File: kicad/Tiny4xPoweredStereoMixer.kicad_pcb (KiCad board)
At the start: 4 copper layers, 99.1 x 56.5 mm, 58 parts, among them J1 AudioJack3_SwitchTR, J2 AudioJack3_SwitchTR, J3 AudioJack3_SwitchTR, J4 AudioJack3_SwitchTR, J6 PowerConnector, J7 PowerConnector, J8 PowerConnector, J9 AudioJack3_SwitchTR, U1 TL072, U2 TL072, U6 LM2611AMF/NOPB

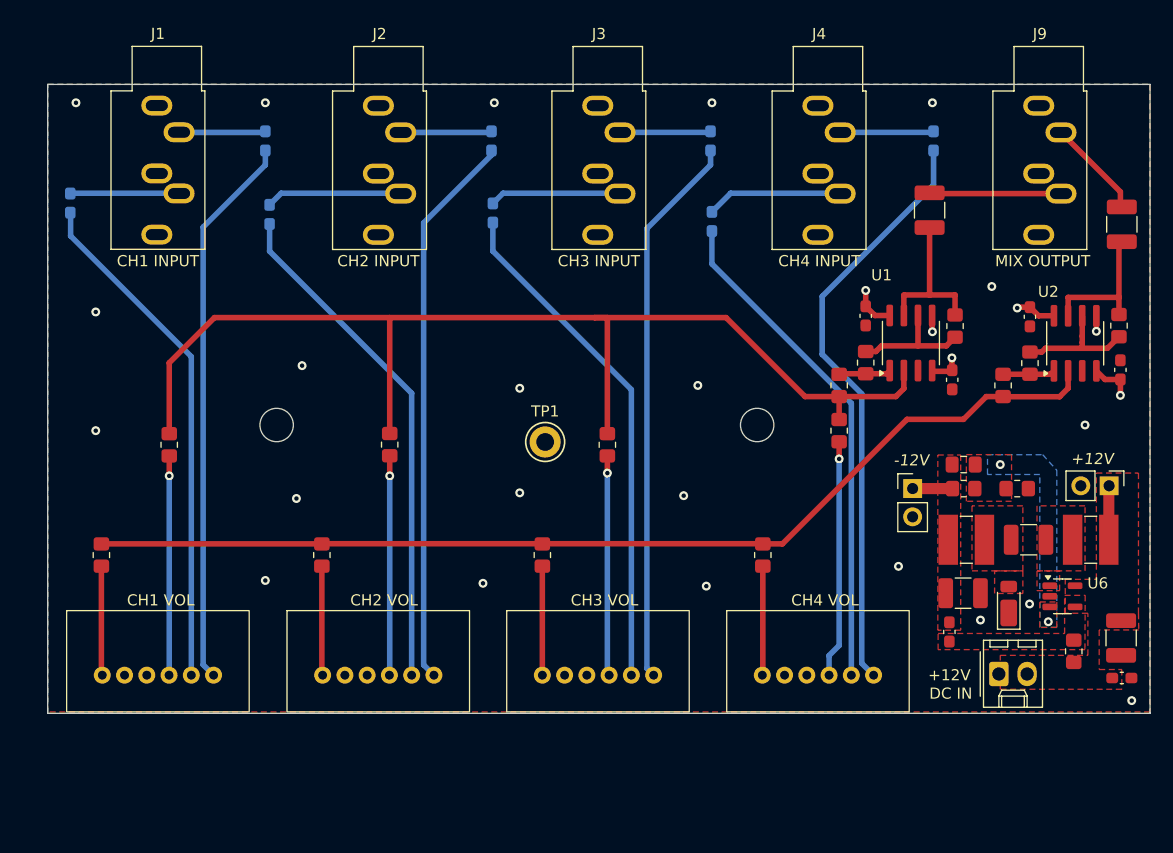
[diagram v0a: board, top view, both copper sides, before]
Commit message: updated main
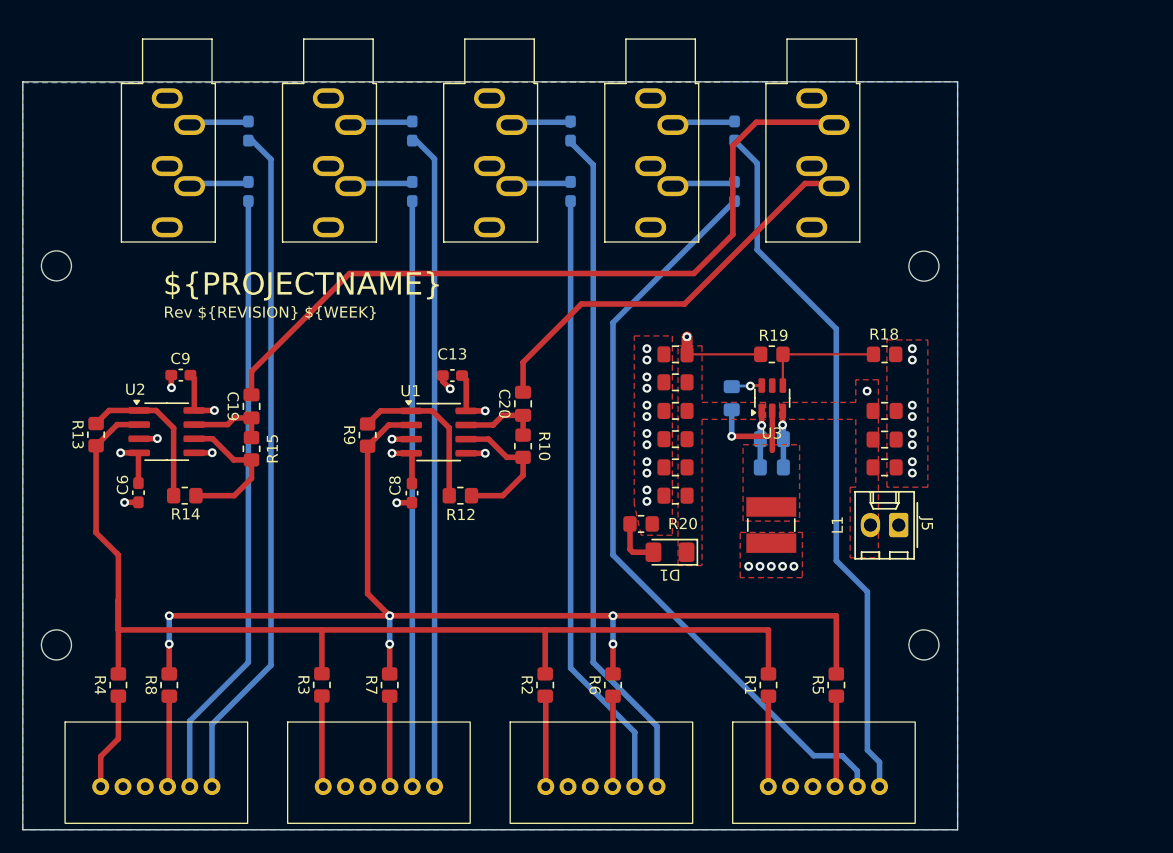
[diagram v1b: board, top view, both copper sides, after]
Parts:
- removed J6: PowerConnector, Connector_Molex:Molex_KK-254_AE-6410-02A_1x02_P2.54mm_Vertical
- removed J7, J8: PowerConnector, Connector_PinHeader_2.54mm:PinHeader_1x02_P2.54mm_Vertical
- removed L2: 22u, Inductor_SMD:L_Ferrocore_DLG-0403
- removed R11: 100k, Resistor_SMD:R_0805_2012Metric_Pad1.20x1.40mm_HandSolder
- removed RFB1: 22k, Resistor_SMD:R_0805_2012Metric_Pad1.20x1.40mm_HandSolder
- removed RFB2: 2k2, Resistor_SMD:R_0805_2012Metric_Pad1.20x1.40mm_HandSolder
- removed TP1: TestPoint, TestPoint:TestPoint_Keystone_5005-5009_Compact
- removed U6: LM2611AMF/NOPB, Package_TO_SOT_SMD:SOT-23-5
- added C21: 100nF, Capacitor_SMD:C_0805_2012Metric_Pad1.18x1.45mm_HandSolder, F.Cu at (160.3, 85.1)
- added C22: 22uF, Capacitor_SMD:C_0805_2012Metric_Pad1.18x1.45mm_HandSolder, F.Cu at (160.3, 87.6)
- added C23: 22uF, Capacitor_SMD:C_0805_2012Metric_Pad1.18x1.45mm_HandSolder, F.Cu at (160.3, 74.9)
- added C24: 22uF, Capacitor_SMD:C_0805_2012Metric_Pad1.18x1.45mm_HandSolder, F.Cu at (160.3, 77.4)
- added C25: 22uF, Capacitor_SMD:C_0805_2012Metric_Pad1.18x1.45mm_HandSolder, F.Cu at (160.3, 80.0)
- added C26: 22uF, Capacitor_SMD:C_0805_2012Metric_Pad1.18x1.45mm_HandSolder, F.Cu at (160.3, 82.5)
- added H3: MountingHole, MountingHole:MountingHole_2.7mm_M2.5, F.Cu at (104.7, 101.0)
- added H4: MountingHole, MountingHole:MountingHole_2.7mm_M2.5, F.Cu at (182.6, 101.0)
- added J5: PowerConnector, Connector_Molex:Molex_KK-254_AE-6410-02A_1x02_P2.54mm_Vertical, F.Cu at (180.4, 90.3)
- added R18: 50K, Resistor_SMD:R_0805_2012Metric_Pad1.20x1.40mm_HandSolder, F.Cu at (179.1, 74.9)
- added R19: 2K4, Resistor_SMD:R_0805_2012Metric_Pad1.20x1.40mm_HandSolder, F.Cu at (169.0, 74.9)
- added R20: 2K2, Resistor_SMD:R_0805_2012Metric_Pad1.20x1.40mm_HandSolder, F.Cu at (157.2, 90.2)
- added U3: TPS54202DDC, Package_TO_SOT_SMD:SOT-23-6, F.Cu at (169.0, 78.9)
- C1: value 22u -> 10uF; footprint Capacitor_SMD:C_1210_3225Metric_Pad1.33x2.70mm_HandSolder -> Capacitor_SMD:C_0805_2012Metric_Pad1.18x1.45mm_HandSolder
- C15: value 100nF -> 10uF; footprint Capacitor_SMD:C_0603_1608Metric_Pad1.08x0.95mm_HandSolder -> Capacitor_SMD:C_0805_2012Metric_Pad1.18x1.45mm_HandSolder; moved to B.Cu
- C16: footprint Capacitor_SMD:C_0603_1608Metric_Pad1.08x0.95mm_HandSolder -> Capacitor_SMD:C_0805_2012Metric_Pad1.18x1.45mm_HandSolder; moved to B.Cu
- C19, C20: footprint Capacitor_SMD:C_1210_3225Metric_Pad1.33x2.70mm_HandSolder -> Capacitor_SMD:C_0805_2012Metric_Pad1.18x1.45mm_HandSolder
- C2: value 2.2u -> 10uF; footprint Capacitor_SMD:C_1210_3225Metric_Pad1.33x2.70mm_HandSolder -> Capacitor_SMD:C_0805_2012Metric_Pad1.18x1.45mm_HandSolder
- C3: value 1n -> 100nF
- C4: value 22u -> 100nF; footprint Capacitor_SMD:C_1210_3225Metric_Pad1.33x2.70mm_HandSolder -> Capacitor_SMD:C_0805_2012Metric_Pad1.18x1.45mm_HandSolder; moved to B.Cu
- D1: value D_Schottky -> LED; footprint Diode_SMD:D_PowerDI-123 -> LED_SMD:LED_1206_3216Metric_Pad1.42x1.75mm_HandSolder
- H1, H2: footprint MountingHole:MountingHole_3mm -> MountingHole:MountingHole_2.7mm_M2.5
- L1: value 22u -> 22uH
- moved U2 82.0 mm to (114.6, 81.9), turned to 0 degrees
- moved R13 81.6 mm to (108.2, 82.1)
- moved C19 79.9 mm to (122.2, 79.6)
- moved R15 78.7 mm to (122.2, 83.4)
- moved R14 76.9 mm to (116.2, 87.6), turned to 0 degrees
- moved C6 73.8 mm to (112.0, 87.4)
- moved C8 64.6 mm to (136.6, 87.4), turned to -90 degrees
- moved C9 61.8 mm to (115.9, 76.8), turned to 180 degrees
- moved C13 52.2 mm to (140.3, 76.8), turned to 180 degrees
- moved U1 43.2 mm to (139.0, 81.9), turned to 0 degrees
- moved R9 42.6 mm to (132.6, 82.2)
- moved C20 40.5 mm to (146.6, 79.4)
- moved R10 40.3 mm to (146.6, 83.2)
- moved R12 38.3 mm to (141.0, 87.6), turned to 0 degrees
- moved C15 38.1 mm to (169.0, 82.5), turned to 180 degrees
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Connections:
- C1 pad 1: GND -> +12V
- C1 pad 2: Net-(J6-Pin_2) -> GND
- C15 pad 1: Net-(J6-Pin_2) -> +12V
- C15 pad 2: GND -> -12V
- C16 pad 1: Net-(J8-Pin_1) -> Net-(U3-BOOT)
- C16 pad 2: Net-(U6-~{SHDN}) -> Net-(U3-SW)
- C2 pad 1: Net-(U6-SW) -> +12V
- C2 pad 2: Net-(D1-A) -> GND
- C3 pad 1: Net-(U6-NFB) -> +12V
- C3 pad 2: Net-(J8-Pin_1) -> GND
- C4 pad 1: GND -> +12V
- C4 pad 2: Net-(J8-Pin_1) -> -12V
- D1 pad 1: GND -> -12V
- L1 pad 1: Net-(J6-Pin_2) -> Net-(U3-SW)
- L1 pad 2: Net-(U6-SW) -> GND
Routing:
- net Net-(C19-Pad2): track 8.96 -> 68.4 mm
- net Net-(C20-Pad2): track 11.7 -> 37.3 mm
- net Net-(C18-Pad2): track 45.1 -> 68.1 mm
- net -12V: track 6.95 -> 22.2 mm, vias 2 -> 4
- net /ch4_right_mix_in: track 21.3 -> 8.52 mm, vias 1 -> 0
- net Net-(C12-Pad2): track 49.8 -> 61.6 mm
- net Net-(C5-Pad2): track 49.8 -> 61.6 mm
- net /ch3_right_mix_in: track 19.8 -> 8.49 mm, vias 1 -> 0
- net /ch2_right_mix_in: track 19.7 -> 8.49 mm, vias 1 -> 0
- net /ch1_right_mix_in: track 19.7 -> 8.54 mm, vias 1 -> 0
- net /TPS54202 Inverting PSU/VSENSE: track 0.00 -> 10.9 mm
- net Net-(C17-Pad2): track 53.2 -> 63.8 mm
- net Net-(R12-Pad1): track 4.68 -> 14.5 mm
- net Net-(U3-SW): track 0.00 -> 9.59 mm, vias 0 -> 1
- net Net-(C14-Pad2): track 45.8 -> 55.4 mm
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- added copper zone on F.Cu, net +12V
- added copper zone on F.Cu, net -12V
- added copper zone on F.Cu, net Net-(U3-SW)
- removed copper zone on F.Cu, net Net-(D1-A)
- removed copper zone on F.Cu, net Net-(J6-Pin_2)
- removed copper zone on F.Cu, net Net-(J8-Pin_1)
- removed copper zone on B.Cu, net Net-(U6-NFB)
- removed copper zone on F.Cu, net Net-(U6-NFB)
- removed copper zone on F.Cu, net Net-(U6-SW)
- removed copper zone on F.Cu, net Net-(U6-~{SHDN})
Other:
- board size 99.1 x 56.5 mm -> 84 x 67.2 mm
- board text added: "${PROJECTNAME}"
- board text added: "Enclosure: https://www.hammfg.com/files/parts/pdf/RM2005S.pdf"
- board text added: "Rev ${REVISION} ${WEEK}"
- board text removed: "Tiny 4-Channel Active Stereo Mixer Rev${REVISION} ${ISSUE_DATE}"

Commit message: changed voltage rails to +/-5V; changed PSU feedback resistor to provide -5V
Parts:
- R19: value 2K4 -> 6K8
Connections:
- net +12V renamed +5V
- net -12V renamed -5V
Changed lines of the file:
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@@
 	(property "WEEK" "43/24")
 	(net 0 "")
-	(net 1 "+12V")
+	(net 1 "+5V")
 	(net 2 "GND")
-	(net 3 "-12V")
+	(net 3 "-5V")
 	(net 4 "Net-(C5-Pad2)")
 	(net 5 "Net-(C5-Pad1)")
@@
 			(layers "F.Cu" "F.Paste" "F.Mask")
 			(roundrect_rratio 0.25)
-			(net 3 "-12V")
+			(net 3 "-5V")
 			(pinfunction "V-")
 			(pintype "power_in")
@@
 			(layers "F.Cu" "F.Paste" "F.Mask")
 			(roundrect_rratio 0.25)
-			(net 1 "+12V")
+			(net 1 "+5V")
 			(pinfunction "V+")
 			(pintype "power_in")
@@
 			(layers "F.Cu" "F.Paste" "F.Mask")
 			(roundrect_rratio 0.212766)
-			(net 1 "+12V")
+			(net 1 "+5V")
 			(pintype "passive")
 		)
@@
 			(layers "F.Cu" "F.Paste" "F.Mask")
 			(roundrect_rratio 0.25)
-			(net 1 "+12V")
+			(net 1 "+5V")
 			(pintype "passive")
 		)
@@
 			(layers "F.Cu" "F.Paste" "F.Mask")
 			(roundrect_rratio 0.25)
-			(net 1 "+12V")
+			(net 1 "+5V")
 			(pintype "passive")
 		)
@@
 			(layers "F.Cu" "F.Paste" "F.Mask")
 			(roundrect_rratio 0.212766)
-			(net 3 "-12V")
+			(net 3 "-5V")
 			(pintype "passive")
 		)
@@
 			(layers "F.Cu" "F.Paste" "F.Mask")
 			(roundrect_rratio 0.212766)
-			(net 3 "-12V")
+			(net 3 "-5V")
 			(pintype "passive")
 		)
@@
 			(layers "F.Cu" "F.Paste" "F.Mask")
 			(roundrect_rratio 0.25)
-			(net 3 "-12V")
+			(net 3 "-5V")
 			(pinfunction "GND")
 			(pintype "power_in")
@@
 			(layers "F.Cu" "F.Paste" "F.Mask")
 			(roundrect_rratio 0.25)
-			(net 1 "+12V")
+			(net 1 "+5V")
 			(pinfunction "VIN")
 			(pintype "power_in")
@@
 			(layers "F.Cu" "F.Paste" "F.Mask")
 			(roundrect_rratio 0.25)
-			(net 3 "-12V")
+			(net 3 "-5V")
 			(pintype "passive")
 		)
@@
 			)
 		)
-		(property "Value" "2K4"
+		(property "Value" "6K8"
 			(at 0 1.65 0)
 			(layer "F.Fab")
@@
 			(layers "F.Cu" "F.Paste" "F.Mask")
 			(roundrect_rratio 0.208333)
-			(net 3 "-12V")
+			(net 3 "-5V")
 			(pintype "passive")
 		)
@@
 			(layers "F.Cu" "F.Paste" "F.Mask")
 			(roundrect_rratio 0.212766)
-			(net 3 "-12V")
+			(net 3 "-5V")
 			(pintype "passive")
 		)
@@
 			(layers "F.Cu" "F.Paste" "F.Mask")
 			(roundrect_rratio 0.212766)
-			(net 1 "+12V")
+			(net 1 "+5V")
 			(pintype "passive")
 		)
@@
 			(layers "F.Cu" "F.Paste" "F.Mask")
 			(roundrect_rratio 0.212766)
-			(net 3 "-12V")
+			(net 3 "-5V")
 			(pintype "passive")
 		)
@@
 			(layers "F.Cu" "F.Paste" "F.Mask")
 			(roundrect_rratio 0.212766)
-			(net 3 "-12V")
+			(net 3 "-5V")
 			(pintype "passive")
 		)
@@
 			(layers "*.Cu" "*.Mask")
 			(remove_unused_layers no)
-			(net 1 "+12V")
+			(net 1 "+5V")
 			(pinfunction "Pin_2")
 			(pintype "passive")
@@
 			)
 		)
-		(property "Mouser" "688-RK12L1210C1K "
+		(property "Mouser" "688-RK12L12A0C0R "
 			(at 0 0 0)
 			(unlocked yes)
@@
 			(layers "F.Cu" "F.Paste" "F.Mask")
 			(roundrect_rratio 0.212766)
-			(net 1 "+12V")
+			(net 1 "+5V")
 			(pintype "passive")
 		)
@@
 			(layers "F.Cu" "F.Paste" "F.Mask")
 			(roundrect_rratio 0.25)
-			(net 3 "-12V")
+			(net 3 "-5V")
 			(pintype "passive")
 		)
@@
 			(layers "F.Cu" "F.Paste" "F.Mask")
 			(roundrect_rratio 0.175439)
-			(net 3 "-12V")
+			(net 3 "-5V")
 			(pinfunction "K")
 			(pintype "passive")
@@
 			)
 		)
-		(property "Mouser" "688-RK12L1210C1K "
+		(property "Mouser" "688-RK12L12A0C0R "
 			(at 0 0 0)
 			(unlocked yes)
@@
 			(layers "F.Cu" "F.Paste" "F.Mask")
 			(roundrect_rratio 0.25)
-			(net 3 "-12V")
+			(net 3 "-5V")
 			(pinfunction "V-")
 			(pintype "power_in")
@@
 			(layers "F.Cu" "F.Paste" "F.Mask")
 			(roundrect_rratio 0.25)
-			(net 1 "+12V")
+			(net 1 "+5V")
 			(pinfunction "V+")
 			(pintype "power_in")
@@
 			)
 		)
-		(property "Mouser" "688-RK12L1210C1K "
+		(property "Mouser" "688-RK12L12A0C0R "
 			(at 0 0 0)
 			(unlocked yes)
@@
 			(layers "F.Cu" "F.Paste" "F.Mask")
 			(roundrect_rratio 0.212766)
-			(net 3 "-12V")
+			(net 3 "-5V")
 			(pintype "passive")
 		)
@@
 			)
 		)
-		(property "Mouser" "688-RK12L1210C1K "
+		(property "Mouser" "688-RK12L12A0C0R "
 			(at 0 0 0)
 			(unlocked yes)
@@
 			(layers "B.Cu" "B.Paste" "B.Mask")
 			(roundrect_rratio 0.212766)
-			(net 1 "+12V")
+			(net 1 "+5V")
 			(pintype "passive")
 		)
@@
 			(layers "B.Cu" "B.Paste" "B.Mask")
 			(roundrect_rratio 0.212766)
-			(net 3 "-12V")
+			(net 3 "-5V")
 			(pintype "passive")
 		)
@@
 			(layers "B.Cu" "B.Paste" "B.Mask")
 			(roundrect_rratio 0.212766)
-			(net 1 "+12V")
+			(net 1 "+5V")
 			(pintype "passive")
 		)
@@
 			(layers "B.Cu" "B.Paste" "B.Mask")
 			(roundrect_rratio 0.212766)
-			(net 3 "-12V")
+			(net 3 "-5V")
 			(pintype "passive")
 		)
@@
 	(zone
 		(net 3)
-		(net_name "-12V")
+		(net_name "-5V")
 		(layer "F.Cu")
 		(hatch edge 0.5)
@@
 	(zone
 		(net 1)
-		(net_name "+12V")
+		(net_name "+5V")
 		(layer "F.Cu")
 		(hatch edge 0.5)
@@
 	(zone
 		(net 1)
-		(net_name "+12V")
+		(net_name "+5V")
 		(layer "In1.Cu")
 		(hatch edge 0.5)
@@
 	(zone
 		(net 3)
-		(net_name "-12V")
+		(net_name "-5V")
 		(layer "In2.Cu")
 		(hatch edge 0.5)

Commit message: Revert "changed voltage rails to +/-5V; changed PSU feedback resistor to provide -5V"
This reverts commit 87719da26a309bbde2d2f76146bcb1e510287c62.
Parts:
- R19: value 6K8 -> 2K4
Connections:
- net +5V renamed +12V
- net -5V renamed -12V
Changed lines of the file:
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@@
 	(property "WEEK" "43/24")
 	(net 0 "")
-	(net 1 "+5V")
+	(net 1 "+12V")
 	(net 2 "GND")
-	(net 3 "-5V")
+	(net 3 "-12V")
 	(net 4 "Net-(C5-Pad2)")
 	(net 5 "Net-(C5-Pad1)")
@@
 			(layers "F.Cu" "F.Paste" "F.Mask")
 			(roundrect_rratio 0.25)
-			(net 3 "-5V")
+			(net 3 "-12V")
 			(pinfunction "V-")
 			(pintype "power_in")
@@
 			(layers "F.Cu" "F.Paste" "F.Mask")
 			(roundrect_rratio 0.25)
-			(net 1 "+5V")
+			(net 1 "+12V")
 			(pinfunction "V+")
 			(pintype "power_in")
@@
 			(layers "F.Cu" "F.Paste" "F.Mask")
 			(roundrect_rratio 0.212766)
-			(net 1 "+5V")
+			(net 1 "+12V")
 			(pintype "passive")
 		)
@@
 			(layers "F.Cu" "F.Paste" "F.Mask")
 			(roundrect_rratio 0.25)
-			(net 1 "+5V")
+			(net 1 "+12V")
 			(pintype "passive")
 		)
@@
 			(layers "F.Cu" "F.Paste" "F.Mask")
 			(roundrect_rratio 0.25)
-			(net 1 "+5V")
+			(net 1 "+12V")
 			(pintype "passive")
 		)
@@
 			(layers "F.Cu" "F.Paste" "F.Mask")
 			(roundrect_rratio 0.212766)
-			(net 3 "-5V")
+			(net 3 "-12V")
 			(pintype "passive")
 		)
@@
 			(layers "F.Cu" "F.Paste" "F.Mask")
 			(roundrect_rratio 0.212766)
-			(net 3 "-5V")
+			(net 3 "-12V")
 			(pintype "passive")
 		)
@@
 			(layers "F.Cu" "F.Paste" "F.Mask")
 			(roundrect_rratio 0.25)
-			(net 3 "-5V")
+			(net 3 "-12V")
 			(pinfunction "GND")
 			(pintype "power_in")
@@
 			(layers "F.Cu" "F.Paste" "F.Mask")
 			(roundrect_rratio 0.25)
-			(net 1 "+5V")
+			(net 1 "+12V")
 			(pinfunction "VIN")
 			(pintype "power_in")
@@
 			(layers "F.Cu" "F.Paste" "F.Mask")
 			(roundrect_rratio 0.25)
-			(net 3 "-5V")
+			(net 3 "-12V")
 			(pintype "passive")
 		)
@@
 			)
 		)
-		(property "Value" "6K8"
+		(property "Value" "2K4"
 			(at 0 1.65 0)
 			(layer "F.Fab")
@@
 			(layers "F.Cu" "F.Paste" "F.Mask")
 			(roundrect_rratio 0.208333)
-			(net 3 "-5V")
+			(net 3 "-12V")
 			(pintype "passive")
 		)
@@
 			(layers "F.Cu" "F.Paste" "F.Mask")
 			(roundrect_rratio 0.212766)
-			(net 3 "-5V")
+			(net 3 "-12V")
 			(pintype "passive")
 		)
@@
 			(layers "F.Cu" "F.Paste" "F.Mask")
 			(roundrect_rratio 0.212766)
-			(net 1 "+5V")
+			(net 1 "+12V")
 			(pintype "passive")
 		)
@@
 			(layers "F.Cu" "F.Paste" "F.Mask")
 			(roundrect_rratio 0.212766)
-			(net 3 "-5V")
+			(net 3 "-12V")
 			(pintype "passive")
 		)
@@
 			(layers "F.Cu" "F.Paste" "F.Mask")
 			(roundrect_rratio 0.212766)
-			(net 3 "-5V")
+			(net 3 "-12V")
 			(pintype "passive")
 		)
@@
 			(layers "*.Cu" "*.Mask")
 			(remove_unused_layers no)
-			(net 1 "+5V")
+			(net 1 "+12V")
 			(pinfunction "Pin_2")
 			(pintype "passive")
@@
 			)
 		)
-		(property "Mouser" "688-RK12L12A0C0R "
+		(property "Mouser" "688-RK12L1210C1K "
 			(at 0 0 0)
 			(unlocked yes)
@@
 			(layers "F.Cu" "F.Paste" "F.Mask")
 			(roundrect_rratio 0.212766)
-			(net 1 "+5V")
+			(net 1 "+12V")
 			(pintype "passive")
 		)
@@
 			(layers "F.Cu" "F.Paste" "F.Mask")
 			(roundrect_rratio 0.25)
-			(net 3 "-5V")
+			(net 3 "-12V")
 			(pintype "passive")
 		)
@@
 			(layers "F.Cu" "F.Paste" "F.Mask")
 			(roundrect_rratio 0.175439)
-			(net 3 "-5V")
+			(net 3 "-12V")
 			(pinfunction "K")
 			(pintype "passive")
@@
 			)
 		)
-		(property "Mouser" "688-RK12L12A0C0R "
+		(property "Mouser" "688-RK12L1210C1K "
 			(at 0 0 0)
 			(unlocked yes)
@@
 			(layers "F.Cu" "F.Paste" "F.Mask")
 			(roundrect_rratio 0.25)
-			(net 3 "-5V")
+			(net 3 "-12V")
 			(pinfunction "V-")
 			(pintype "power_in")
@@
 			(layers "F.Cu" "F.Paste" "F.Mask")
 			(roundrect_rratio 0.25)
-			(net 1 "+5V")
+			(net 1 "+12V")
 			(pinfunction "V+")
 			(pintype "power_in")
@@
 			)
 		)
-		(property "Mouser" "688-RK12L12A0C0R "
+		(property "Mouser" "688-RK12L1210C1K "
 			(at 0 0 0)
 			(unlocked yes)
@@
 			(layers "F.Cu" "F.Paste" "F.Mask")
 			(roundrect_rratio 0.212766)
-			(net 3 "-5V")
+			(net 3 "-12V")
 			(pintype "passive")
 		)
@@
 			)
 		)
-		(property "Mouser" "688-RK12L12A0C0R "
+		(property "Mouser" "688-RK12L1210C1K "
 			(at 0 0 0)
 			(unlocked yes)
@@
 			(layers "B.Cu" "B.Paste" "B.Mask")
 			(roundrect_rratio 0.212766)
-			(net 1 "+5V")
+			(net 1 "+12V")
 			(pintype "passive")
 		)
@@
 			(layers "B.Cu" "B.Paste" "B.Mask")
 			(roundrect_rratio 0.212766)
-			(net 3 "-5V")
+			(net 3 "-12V")
 			(pintype "passive")
 		)
@@
 			(layers "B.Cu" "B.Paste" "B.Mask")
 			(roundrect_rratio 0.212766)
-			(net 1 "+5V")
+			(net 1 "+12V")
 			(pintype "passive")
 		)
@@
 			(layers "B.Cu" "B.Paste" "B.Mask")
 			(roundrect_rratio 0.212766)
-			(net 3 "-5V")
+			(net 3 "-12V")
 			(pintype "passive")
 		)
@@
 	(zone
 		(net 3)
-		(net_name "-5V")
+		(net_name "-12V")
 		(layer "F.Cu")
 		(hatch edge 0.5)
@@
 	(zone
 		(net 1)
-		(net_name "+5V")
+		(net_name "+12V")
 		(layer "F.Cu")
 		(hatch edge 0.5)
@@
 	(zone
 		(net 1)
-		(net_name "+5V")
+		(net_name "+12V")
 		(layer "In1.Cu")
 		(hatch edge 0.5)
@@
 	(zone
 		(net 3)
-		(net_name "-5V")
+		(net_name "-12V")
 		(layer "In2.Cu")
 		(hatch edge 0.5)
